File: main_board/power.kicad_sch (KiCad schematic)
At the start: 29 parts, among them J10 B5B-XH, J11 B5B-XH, J12 B3B-XH, J13 B5B-XH, J8 Conn_01x02, J9 Conn_01x02, Q10 DTC114E, Q9 DTC114E, U12 OKL-T/6-W12N-C, U13 XC6221B302GR, U14 FT232RL, U15 SL2.1A, Y1 12MHz

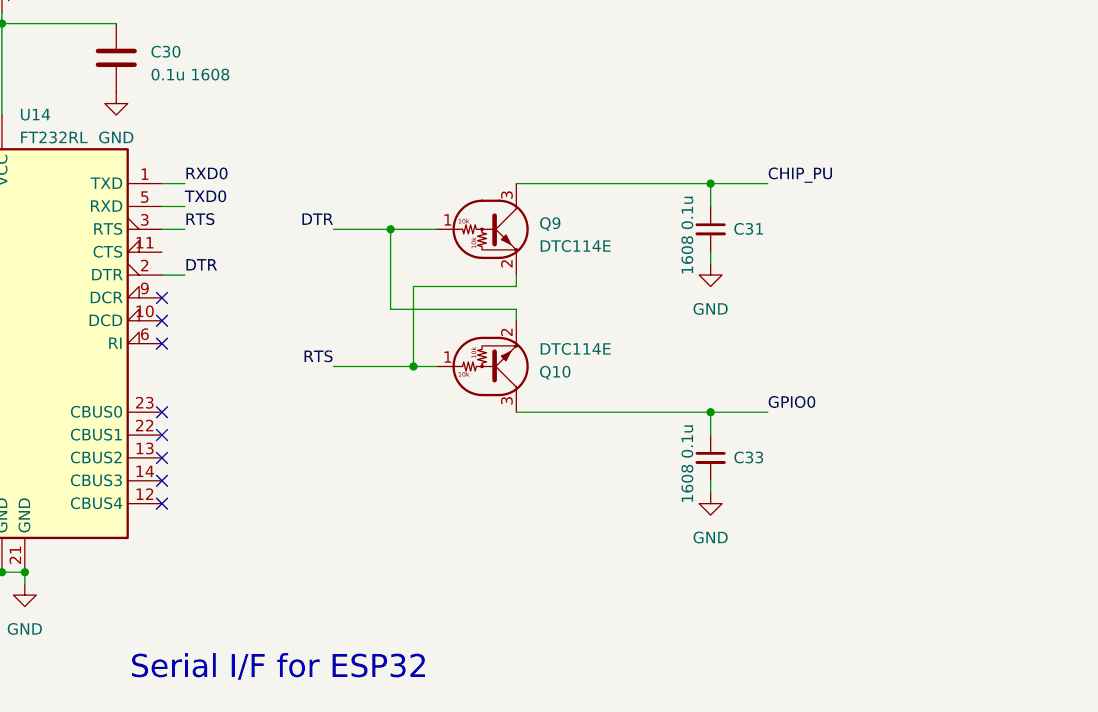
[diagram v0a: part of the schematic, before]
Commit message: アートワーク : 部品配置
Signed-off-by: Kazuki Iida <elkel53930@gmail.com>
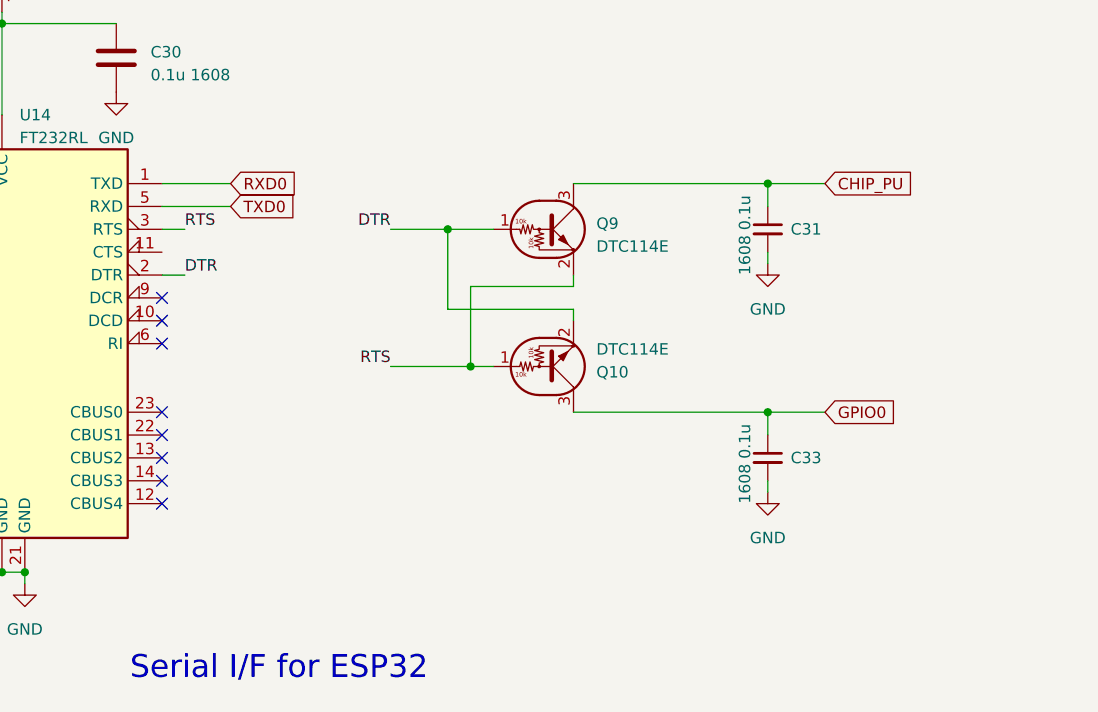
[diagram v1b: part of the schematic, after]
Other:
- moved on the sheet: C31, C33, Q10, Q9
